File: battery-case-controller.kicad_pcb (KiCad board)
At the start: 6 copper layers, 110 x 55 mm, 187 parts, among them J31 +, J32 Display, J33 A, J34 HALL, J35 B, J36 MOT_AUX, J37 C, J38 CRANK, J39 GND, J40 CAN_IN, J41 CAN_OUT, J42 Debug, J43 SWD, M31 MountingHole_Pad, M32 MountingHole_Pad, M33 MountingHole_Pad, Q31 BSC040N08, Q32 BSC040N08, Q33 BSC040N08, Q34 BSC040N08, Q35 BSC040N08, Q36 BSC040N08, Q37 BSC040N08, Q38 BSC040N08, Q39 BSC040N08, Q40 BSC040N08, Q41 BSC040N08, Q42 BSC040N08, U31 Enable, U32 LM5109B, U33 INA240A2PWR, U34 LM5109B, U35 INA240A2PWR, U36 LM5109B, U37 INA240A2PWR, U38 LM5008, U39 XC6206P332MR, U40 XC6206P332MR, U41 LMR12010X, U42 SN65HVD230, U43 STM32G491CxT, X31 8MHz

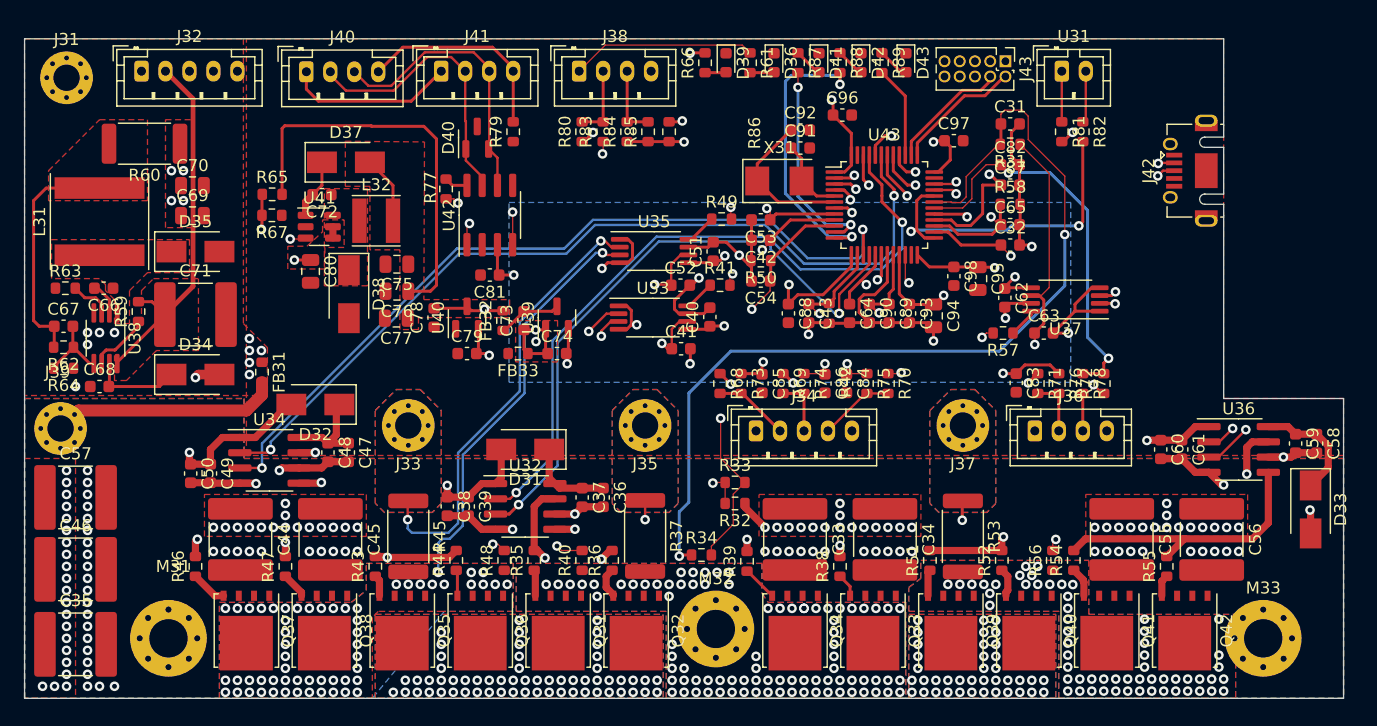
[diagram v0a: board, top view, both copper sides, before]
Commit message: Ordered
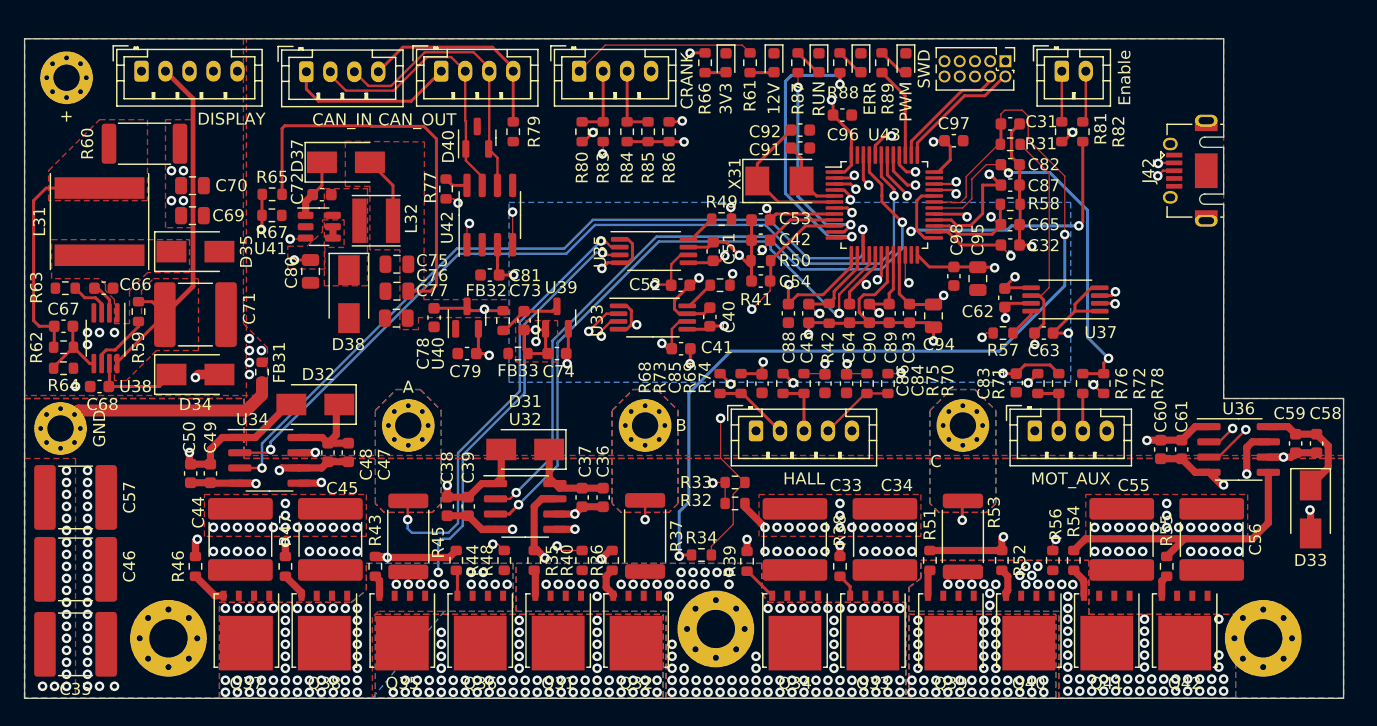
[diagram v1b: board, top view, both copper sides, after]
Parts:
- D42: value ERROR -> ERR
- J32: value Display -> DISPLAY
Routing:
- net GNDA: track 101.3 -> 96.7 mm
- net +12V: track 131.8 -> 128.5 mm
- net Net-(R65-Pad1): track 7.53 -> 7.01 mm
- net Net-(C36-Pad2): vias 87 -> 86
